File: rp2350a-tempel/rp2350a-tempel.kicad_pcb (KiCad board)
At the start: 2 copper layers, 36 parts, among them J1 Conn_North, J2 Conn_East, J3 Conn_South, J4 Conn_West, SW1 BOOT SELECTOR, SW2 RST, U1 AMS1117-3.3, U2 W25Q16JVSS, U3 RP2350_60QFN, Y1 12Mhz HC49-SD

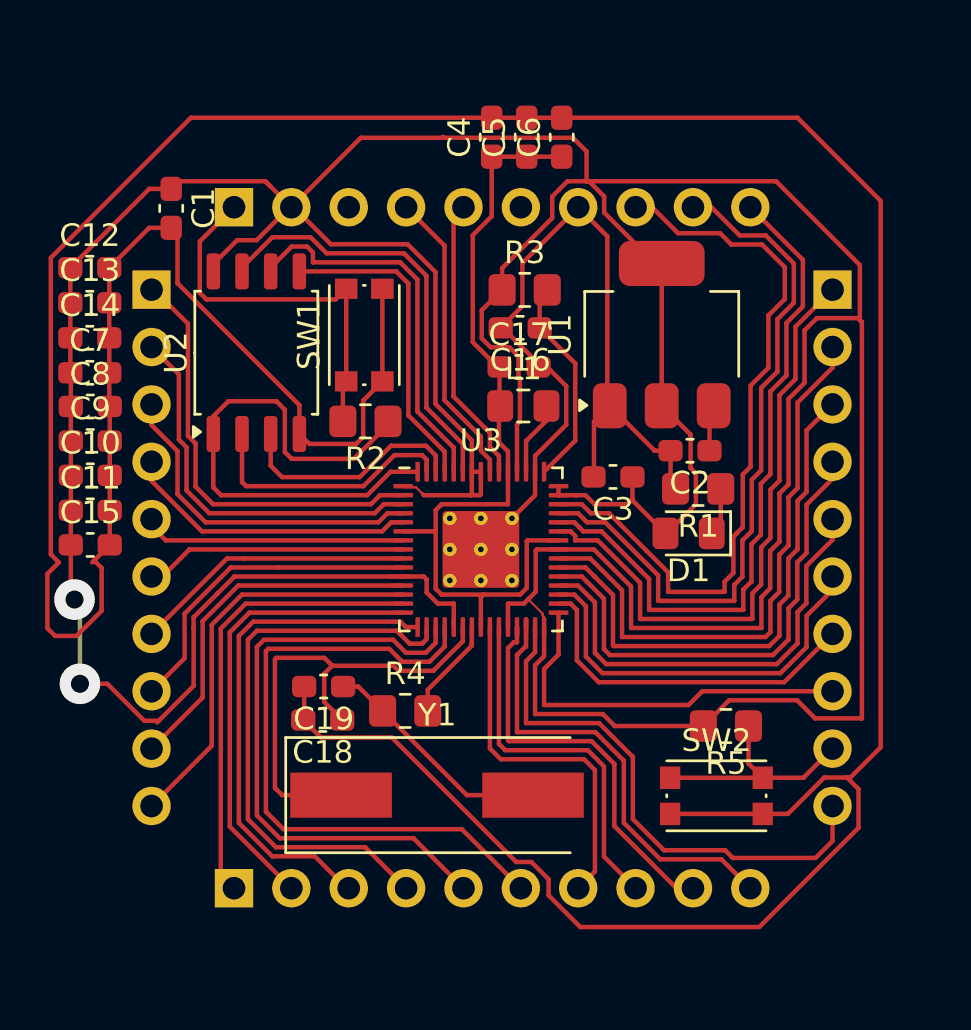
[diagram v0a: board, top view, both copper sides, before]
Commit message: feat: finish routing
Update README.md
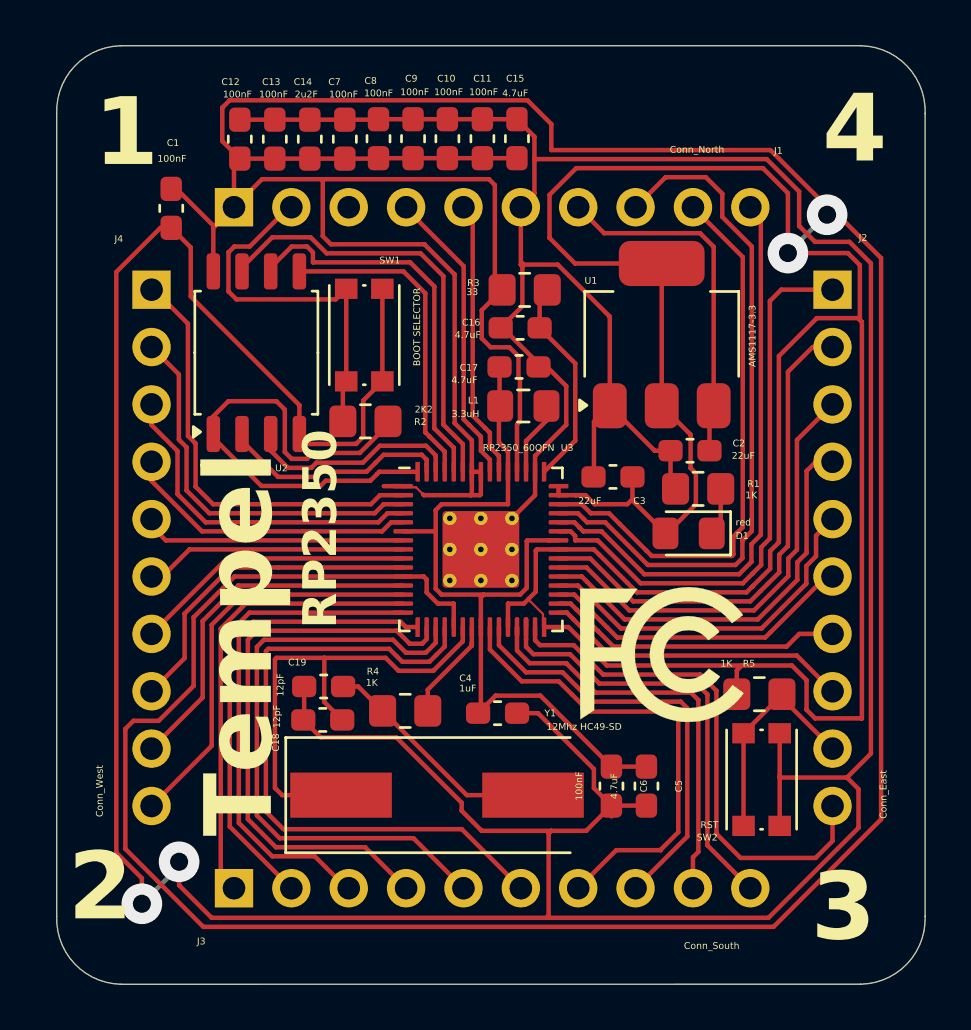
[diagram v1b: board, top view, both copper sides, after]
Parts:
- added REF**: FCC-Logo_7.3x6mm_SilkScreen, Symbol:FCC-Logo_7.3x6mm_SilkScreen, F.Cu at (144.8, 77.3)
- L1: value L -> 3.3uH
- moved C5 29.2 mm to (144.1, 83.1), turned to -90 degrees
- moved C6 28.8 mm to (142.6, 83.1), turned to -90 degrees
- moved C15 26.1 mm to (138.4, 54.5), turned to 90 degrees
- moved C4 25.5 mm to (137.5, 79.9), turned to 0 degrees
- moved C11 23.9 mm to (136.8, 54.5), turned to 90 degrees
- moved C10 21.7 mm to (135.3, 54.5), turned to 90 degrees
- moved C9 19.6 mm to (133.8, 54.5), turned to 90 degrees
- moved C8 17.4 mm to (132.2, 54.5), turned to 90 degrees
- moved C7 15.3 mm to (130.8, 54.5), turned to 90 degrees
- moved C14 13.1 mm to (129.2, 54.5), turned to 90 degrees
- moved C13 10.9 mm to (127.7, 54.5), turned to 90 degrees
- moved C12 8.75 mm to (126.1, 54.5), turned to 90 degrees
- moved SW2 2.13 mm to (149.2, 82.8), turned to 90 degrees
- moved R5 2.04 mm to (149.1, 79.1)
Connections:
- J1 pad 1: /~{BOOTSEL} -> +3.3V
- J1 pad 2: +3.3V -> /~{BOOTSEL}
- J1 pad 6: +5V -> GND
- J1 pad 7: GND -> +5V
- J1 pad 8: /GPIO29_ADC3 -> /GPIO28_ADC2
- J1 pad 9: /GPIO28_ADC2 -> /GPIO29_ADC3
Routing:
- net +3.3V: track 228.9 -> 313.0 mm
- net GND: track 206.4 -> 220.9 mm, vias 0 -> 2
- net +5V: track 2.07 -> 15.8 mm
- net /GPIO29_ADC3: track 32.7 -> 25.2 mm
- net /SWCLK: track 16.0 -> 21.2 mm
- net /GPIO27_ADC1: track 30.5 -> 25.8 mm
- net /GPIO22: track 19.9 -> 15.9 mm
- net /GPIO24: track 23.9 -> 20.0 mm
- net /GPIO19: track 17.4 -> 13.6 mm
- net /GPIO21: track 17.8 -> 14.0 mm
- net /GPIO23: track 21.9 -> 18.4 mm
- net /GPIO25: track 25.9 -> 22.6 mm
- net /SWD: track 16.2 -> 19.2 mm
- net /GPIO20: track 15.8 -> 13.2 mm
- net /GPIO26_ADC0: track 27.3 -> 25.2 mm
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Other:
- board outline added: 38.4 x 41.6 mm
- board text added: "1"
- board text added: "2"
- board text added: "3"
- board text added: "4"
- board text added: "RP2350"
- board text added: "Tempel"
